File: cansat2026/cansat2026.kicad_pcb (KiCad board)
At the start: 6 copper layers, 96 x 70 mm, 282 parts, among them J101 MCU_UART_Conn, J102 CAM_Conn, J103 MCU_CAM_UART_Conn, J104 I2C_Conn, J105 MCU_Power, J106 MCU_Power, J107 Micro_SD_Card_Det_Hirose_DM3AT, J1101 USB_C_Receptacle_USB2.0_14P, J1102 USB_C_Receptacle_USB2.0_14P, J201 FlightPin, J301 Battery, J302 Battery, J401 M1, J402 M2, J403 M3, J801 Conn_Coaxial, Q1101 2N7002, Q1102 2N7002, Q1103 2N7002, Q1104 2N7002, Q301 2SB1198K, Q302 2SB1198K, Q303 2N7002, Q304 2SB1198K, Q305 2N7002, Q306 2SC2412K, Q307 PJA3404A, Q308 PJA3404A, SW201 SW_SPST, SW901 SW_SPST, U1001 ICE40UP5K-SG48ITR, U101 E220-900T22S(JP), U1101 USBLC6-2SC6, U1102 CH340K, U1103 USBLC6-2SC6, U1104 CH340K, U201 TPS70912DRVR, U202 TCR2LN18, U203 TPS561201DDC, U204 74HC08, U205 INA226, U206 TPS562242, U207 XC6206P332MR, U208 TPS62180, U209 TPS62180, U210 TPS63070, U301 S-8209ABB-T8T1U, U302 S-8209ABB-T8T1U, U401 TC78H653FTG, U402 TC78H653FTG, U403 AM8068, U601 HP203B, U701 LSM6DSV, U801 MAX-M10S, U901 ESP32-S3-WROOM-1U-N4R8, U902 ESP32-S3-WROOM-1U-N4R8, U903 AW9523B, U904 PCA9306DQER, U905 PCA9306DQER

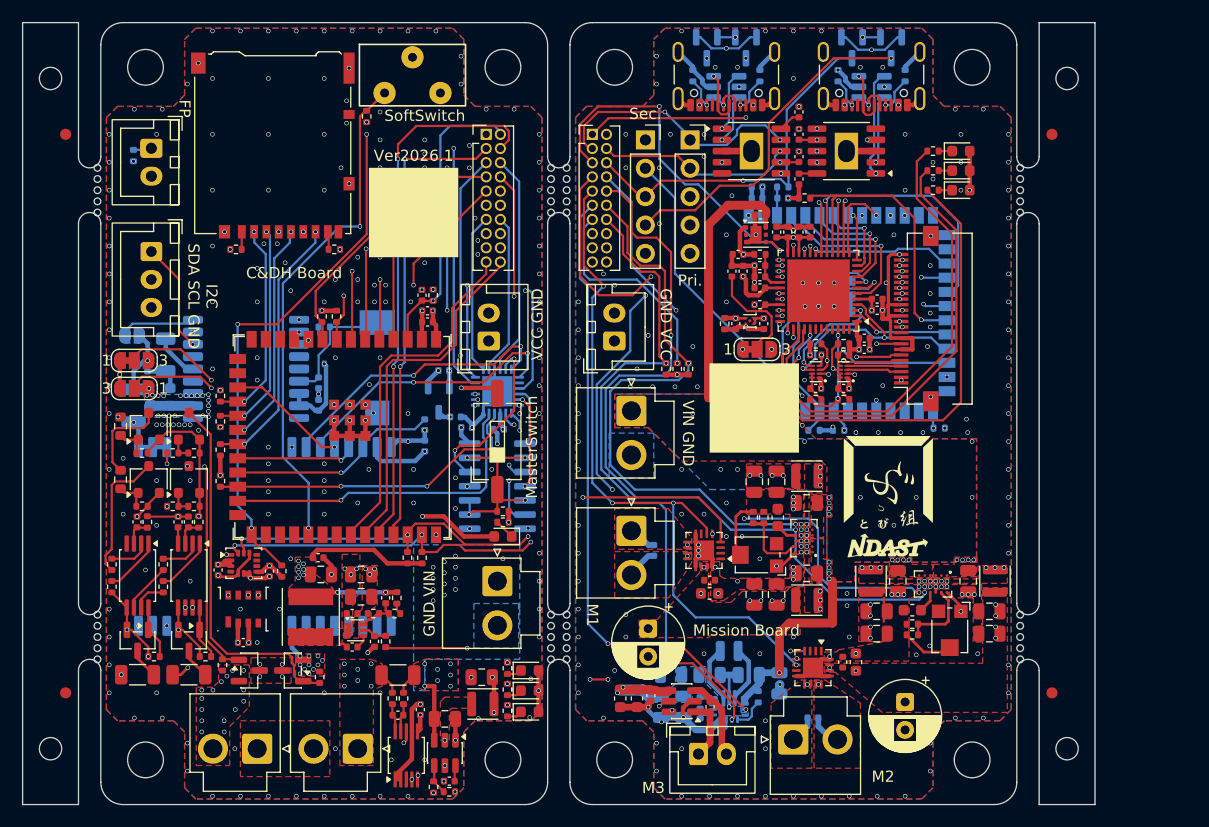
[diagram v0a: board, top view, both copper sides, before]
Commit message: ARLISSに作り直した
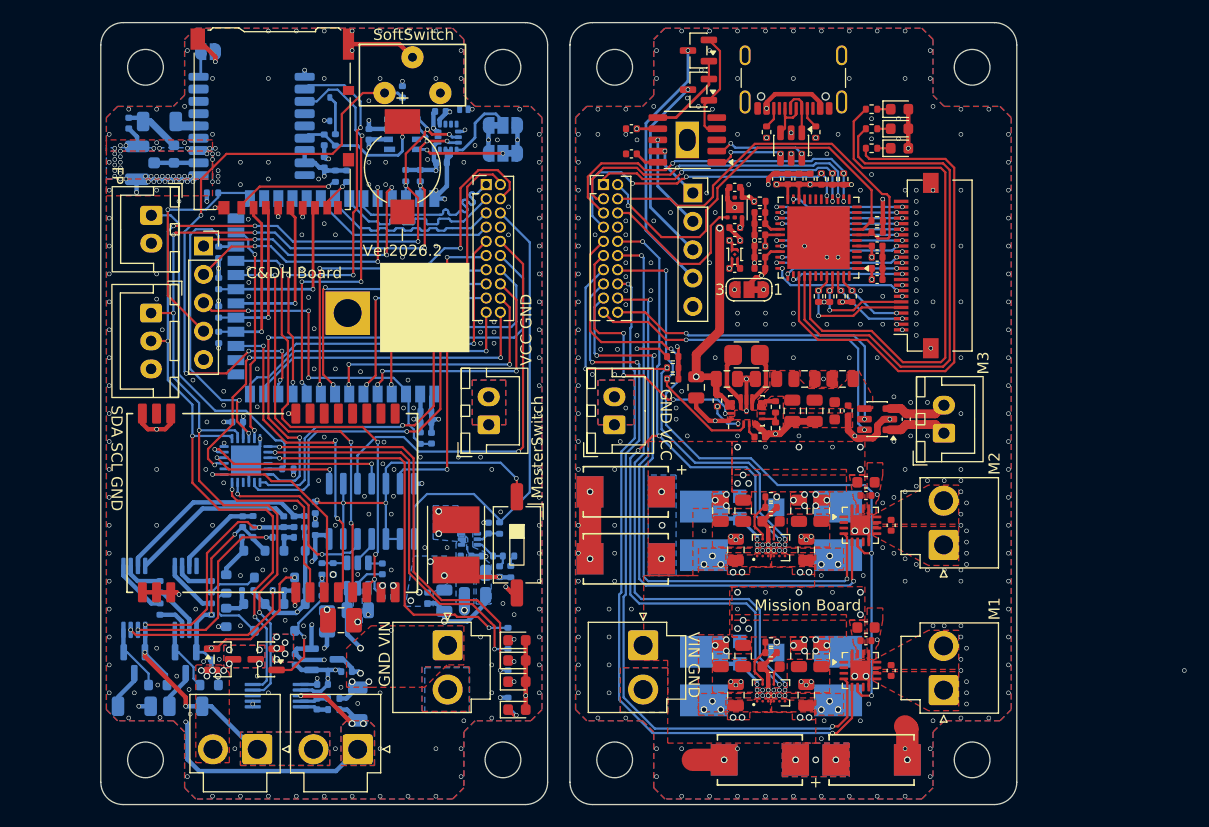
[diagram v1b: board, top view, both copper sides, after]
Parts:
- removed C1103, C1104, C908, C909: 100nF, Capacitor_SMD:C_0402_1005Metric
- removed the C903 at (98.7, 35.5)
- removed the C904 at (98.7, 34.5)
- removed C905: 1uF, Capacitor_SMD:C_0402_1005Metric
- removed the J103 at (88.7, 30.2)
- removed J1102: USB_C_Receptacle_USB2.0_14P, Connector_USB:USB_C_Receptacle_GCT_USB4105-xx-A_16P_TopMnt_Horizontal
- removed Q1103, Q1104: 2N7002, Package_TO_SOT_SMD:SOT-23
- removed R1103, R1104: 5.1k, Resistor_SMD:R_0402_1005Metric
- removed the R901 at (101.0, 34.5)
- removed the R905 at (115.0, 56.0)
- removed the R909 at (59.8, 46.0)
- removed the R917 at (103.0, 35.5)
- removed the R918 at (106.5, 53.5)
- removed the R919 at (95.8, 46.7)
- removed R923: 200k, Resistor_SMD:R_0402_1005Metric
- removed the REF** at (126.5, 24.8)
- removed the REF** at (125.1, 79.8)
- removed the REF** at (36.8, 29.8)
- removed the REF** at (125.1, 29.8)
- removed the REF** at (80.0, 74.8)
- removed the REF** at (40.0, 34.8)
- removed the REF** at (80.0, 34.8)
- removed the REF** at (36.8, 79.8)
- removed the REF** at (122.0, 34.8)
- removed the REF** at (35.5, 84.8)
- removed the REF** at (40.0, 74.8)
- removed the REF** at (126.5, 84.8)
- removed the REF** at (35.5, 24.8)
- removed the REF** at (122.0, 74.8)
- removed U1103: USBLC6-2SC6, Package_TO_SOT_SMD:SOT-23-6
- removed U1104: CH340K, Package_SO:SSOP-10-1EP_3.9x4.9mm_P1mm_EP2.1x3.3mm
- removed the U902 at (106.2, 45.8)
- removed U904, U905: PCA9306DQER, Package_SON:X2SON-8_1.4x1mm_P0.35mm
- added C413: 100uF, Project:MURATA_ECAS_D6, B.Cu at (99.0, 85.8)
- added C414: 100uF, Project:MURATA_ECAS_D6, F.Cu at (87.0, 61.8)
- added C415: 100uF, Project:MURATA_ECAS_D6, B.Cu at (87.0, 61.8)
- added C416: 100uF, Project:MURATA_ECAS_D6, F.Cu at (87.0, 67.8)
- added C417: 100uF, Project:MURATA_ECAS_D6, B.Cu at (87.0, 67.8)
- added C418: 22uF, Capacitor_SMD:C_0805_2012Metric, F.Cu at (106.4, 51.6)
- added J101: MCU_UART_Conn, Connector_PinSocket_2.54mm:PinSocket_1x05_P2.54mm_Vertical, F.Cu at (49.2, 39.8)
- added R906: 10k, Resistor_SMD:R_0402_1005Metric, F.Cu at (105.5, 33.8)
- added R907: 10k, Resistor_SMD:R_0402_1005Metric, F.Cu at (104.5, 33.8)
- BT801, C235, C236, C237, C238, C239, C240, C241, C403, C406, Q1101, Q1102, R1002, R1003, R1101, R1102, R220, R221, R222, U101, U1101, U210: moved to F.Cu
- C205, C206, C207, C209, C210, C211, C212, C213, C214, C215, C216, C217, C218, C301, C302, C303, C601, C701, C702, C901, C902, G*** (x2), JP601, JP701, Q301, Q302, Q303, Q304, Q305, Q306, R101, R102, R202, R203, R204, R205, R206, R207, R208, R209, R210, R211, R218, R301, R302, R303, R304, R305, R306, R308, R309, R310, R311, R312, R313, R315, R316, R317, R318, R319, R320, RV201, RV202, U203, U205, U206, U301, U302, U601, U701, U901: moved to B.Cu
- C410: footprint Capacitor_THT:CP_Radial_D6.3mm_P2.50mm -> Project:MURATA_ECAS_D6
- C411: footprint Capacitor_THT:CP_Radial_D6.3mm_P2.50mm -> Project:MURATA_ECAS_D6; moved to B.Cu
- C412: value 10uF -> 100uF; footprint Capacitor_SMD:C_0603_1608Metric -> Project:MURATA_ECAS_D6
- C903: renamed from C906; moved to B.Cu
- L201: footprint Inductor_SMD:L_Wuerth_PMCI-252012 -> Inductor_SMD:L_1008_2520Metric_Pad1.43x2.20mm_HandSolder
- L202: footprint Inductor_SMD:L_Taiyo-Yuden_NR-50xx -> Inductor_SMD:L_Taiyo-Yuden_NR-50xx_HandSoldering
- L203, L204, L205, L206: footprint Inductor_SMD:L_Wuerth_PMCI-252010 -> Project:L_Taiyo-Yuden_LSEU-4040; moved to B.Cu
- L207: footprint Inductor_SMD:L_Wuerth_PMCI-201610 -> Project:L_Wuerth_PMCI-201610; moved to F.Cu
- R307, R314: footprint Resistor_SMD:R_0402_1005Metric -> Resistor_SMD:R_0603_1608Metric; moved to B.Cu
- R901: renamed from R902; moved to B.Cu
- R902: renamed from R903; moved to B.Cu
- R903: renamed from R904; moved to B.Cu
- R904: renamed from R906; moved to B.Cu
- R905: renamed from R907; moved to B.Cu
- R908: value 4.7k -> 10k
- R909: renamed from R911; moved to B.Cu
- R910: renamed from R912; moved to B.Cu
- R911: renamed from R913; moved to B.Cu
- R914: renamed from R910; moved to B.Cu
- R917: renamed from R914; moved to B.Cu
- R918: renamed from R915; moved to B.Cu
- R919: renamed from R916; moved to B.Cu
- moved R908 47.0 mm to (106.5, 33.8), turned to 90 degrees
- moved C601 46.9 mm to (64.0, 29.8), turned to -90 degrees
- moved U601 44.8 mm to (67.0, 29.8), turned to 90 degrees
- moved C702 43.9 mm to (70.4, 27.7), turned to 180 degrees
- moved U701 42.3 mm to (71.1, 30.0), turned to 90 degrees
- moved C701 41.6 mm to (70.5, 32.3), turned to 0 degrees
- moved JP601 39.1 mm to (76.0, 31.4)
- moved JP701 39.1 mm to (76.0, 28.9)
- moved J403 36.2 mm to (115.4, 56.5), turned to 90 degrees
- moved R903 34.4 mm to (50.0, 35.0), turned to 0 degrees
- moved R904 34.2 mm to (68.6, 33.5), turned to -90 degrees
- moved R905 34.2 mm to (67.3, 33.5), turned to -90 degrees
- moved J401 31.4 mm to (115.4, 79.5), turned to 90 degrees
- moved R201 31.3 mm to (56.7, 59.7), turned to 180 degrees
- moved C407 31.2 mm to (105.7, 54.5)
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- renumbered C907 to C904, J104 to J103, J105 to J104, J106 to J105, J107 to J106, R920 to R912, R921 to R913, R924 to R915, R925 to R916, U903 to U902
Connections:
- C1011 pad 1: /VCC -> Net-(JP1001-C)
- C1012 pad 1: /VCC -> Net-(JP1001-C)
- C411 pad 1: /MD/M2PWR -> /MD/M1PWR
- C412 pad 1: /MD/M3PWR -> /MD/M1PWR
- R908 pad 2: /MCU/I2C2SDA -> /MCU/FPGA_SPI_MISO
- R912 pad 2: /MCU/CP_CAM_PIN_SIOC -> /CAM_PIN_SIOC
- R913 pad 2: /MCU/CP_CAM_PIN_SIOD -> /CAM_PIN_SIOD
- REF** pad 1: /GPIO0 -> /MCU/FPGA_SPI_SS (x2)
- REF** pad 2: /EN -> /MCU/FPGA_~{CRESET} (x2)
- REF** pad 3: /U0TXD -> /MCU/FPGA_SPI_SCK (x2)
- REF** pad 4: /U0RXD -> /MCU/FPGA_CDONE (x2)
- REF** pad 5: /Power/MASTER_EN -> /MCU/FPGA_SPI_MISO (x2)
- REF** pad 6: /MCU_CAM_EN -> /Power/MASTER_EN (x2)
- REF** pad 7: /MCU/I2C2SCL -> /MCU/FPGA_SPI_MOSI (x2)
- REF** pad 8: /MCU/I2C2SDA -> (no net) (x2)
- U1001 pad 1: /VCC -> Net-(JP1001-C)
- U1001 pad 10: /MCU/CP_CAM_PIN_D2 -> unconnected-(U1001B-IOB_18a-Pad10)
- U1001 pad 11: /MCU/CP_CAM_PIN_D3 -> unconnected-(U1001B-IOB_20a-Pad11)
- U1001 pad 12: /MCU/CP_CAM_PIN_D4 -> unconnected-(U1001B-IOB_22a-Pad12)
- U1001 pad 13: /MCU/CP_CAM_PIN_D6 -> unconnected-(U1001B-IOB_24a-Pad13)
- U1001 pad 18: /MCU/CP_CAM_PIN_D7 -> unconnected-(U1001B-IOB_31b-Pad18)
- U1001 pad 19: /MCU/CP_CAM_PIN_HREF -> unconnected-(U1001B-IOB_29b-Pad19)
- U1001 pad 2: /MCU/CP_CAM_PIN_VSYNC -> unconnected-(U1001C-IOB_6a-Pad2)
- U1001 pad 20: /MCU/CP_CAM_PIN_PCLK -> unconnected-(U1001B-IOB_25b_G3-Pad20)
- U1001 pad 21: /MCU/CP_CAM_PIN_D5 -> unconnected-(U1001B-IOB_23b-Pad21)
- U1001 pad 3: /MCU/CP_CAM_PIN_RESET -> unconnected-(U1001C-IOB_9b-Pad3)
- U1001 pad 4: /MCU/CP_CAM_PIN_PWDN -> unconnected-(U1001C-IOB_8a-Pad4)
- U1001 pad 44: unconnected-(U1001C-IOB_3b_G6-Pad44) -> /CAM_PIN_PWDN
- U1001 pad 45: unconnected-(U1001C-IOB_5b-Pad45) -> /CAM_PIN_RESET
- U1001 pad 46: /MCU/LS_EN -> /CAM_PIN_SIOC
- U1001 pad 47: unconnected-(U1001C-IOB_2a-Pad47) -> /CAM_PIN_SIOD
- U1001 pad 6: /MCU/CP_CAM_PIN_D0 -> unconnected-(U1001B-IOB_13b-Pad6)
- U1001 pad 9: /MCU/CP_CAM_PIN_D1 -> unconnected-(U1001B-IOB_16a-Pad9)
- U210 pad : VIN -> (no net)
- U801 pad 16: /I2C1SDA -> unconnected-(U801-SDA-Pad16)
- U801 pad 17: /I2C1SCL -> unconnected-(U801-SCL-Pad17)
- U901 pad 12: unconnected-(U901-GPIO8/TOUCH8/ADC1_CH7/SUBSPICS1-Pad12) -> /MCU/SW_SOFT
- U901 pad 13: unconnected-(U901-GPIO19/U1RTS/ADC2_CH8/CLK_OUT2/USB_D--Pad13) -> /MCU/MC2
- U901 pad 14: unconnected-(U901-GPIO20/U1CTS/ADC2_CH9/CLK_OUT1/USB_D+-Pad14) -> /MCU/MC1
- U901 pad 31: /MCU/SW_SOFT -> unconnected-(U901-GPIO38/FSPIWP/SUBSPIWP-Pad31)
- U901 pad 32: unconnected-(U901-MTCK/GPIO39/CLK_OUT3/SUBSPICS1-Pad32) -> /MCU/FPGA_SPI_MOSI
- U901 pad 33: unconnected-(U901-MTDO/GPIO40/CLK_OUT2-Pad33) -> /MCU/FPGA_SPI_MISO
- U901 pad 34: /MCU/MC1 -> /MCU/FPGA_SPI_SCK
- U901 pad 35: /MCU/MC2 -> /MCU/FPGA_SPI_SS
- U901 pad 8: /MCU/I2C2SDA -> /MCU/FPGA_~{CRESET}
- U901 pad 9: /MCU/I2C2SCL -> /MCU/FPGA_CDONE
- U902 pad 10: /MCU_CAM_EN -> unconnected-(U902-P0_4-Pad10)
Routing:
- net GND: track 225.1 -> 419.4 mm, vias 434 -> 573
- net /MCU_CAM_GPIO0: track 67.8 -> 0.00 mm, vias 2 -> 0
- net /MCU/I2C2SCL: track 60.2 -> 0.00 mm, vias 2 -> 0
- net /MCU/I2C2SDA: track 57.4 -> 0.00 mm, vias 4 -> 0
- net /MCU_CAM_EN: track 53.1 -> 0.00 mm, vias 1 -> 0
- net /MCU/FPGA_CDONE: track 22.4 -> 73.7 mm, vias 1 -> 3
- net /MCU_CAM_U0RXD: track 51.0 -> 0.00 mm, vias 2 -> 0
- net /MCU/FPGA_~{CRESET}: track 26.4 -> 72.3 mm, vias 3 -> 4
- net /GPIO0: track 89.4 -> 44.4 mm, vias 5 -> 2
- net /MCU_CAM_U0TXD: track 43.7 -> 0.00 mm, vias 2 -> 0
- net Net-(U210-EN): track 90.3 -> 52.7 mm, vias 5 -> 6
- net /GPS/GPS_TX: track 0.83 -> 38.2 mm, vias 1 -> 4
- net /GPS/GPS_RX: track 0.99 -> 37.1 mm, vias 1 -> 4
- net /3.8V: track 45.5 -> 9.46 mm, vias 4 -> 3
- net /U0TXD: track 65.2 -> 29.3 mm
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- added copper zone on In2.Cu, net /1.2V
- added copper zone on B.Cu, net /MD/M1PWR
- added copper zone on B.Cu, net /MD/M2PWR
- added copper zone on F.Cu, net /MD/M3PWR
- added copper zone on B.Cu, net /Power/BATT+
- added copper zone on In1.Cu, net /Power/BATT+
- added copper zone on B.Cu, net /VCC
- added copper zone on B.Cu, net Net-(J301-Pin_2)
- added copper zone on In1.Cu, net Net-(J301-Pin_2)
- added copper zone on In2.Cu, net Net-(J302-Pin_2)
- added copper zone on In2.Cu, net Net-(JP1001-C)
- added copper zone on B.Cu, net Net-(Q307-D)
- added copper zone on In2.Cu, net Net-(Q307-D)
- added copper zone on B.Cu, net Net-(U203-SW)
- added copper zone on B.Cu, net Net-(U206-SW)
- removed copper zone on In3.Cu, net /MD/M1PWR
- removed copper zone on In3.Cu, net /MD/M2PWR
- removed copper zone on B.Cu, net /MD/M3PWR
- removed copper zone on F.Cu, net /VCC
- removed copper zone on In3.Cu, net GND
- removed copper zone on In4.Cu, net GND
- removed copper zone on In4.Cu, net Net-(J301-Pin_2)
- removed copper zone on In2.Cu, net Net-(J401-Pin_1)
- removed copper zone on In2.Cu, net Net-(J401-Pin_2)
- removed copper zone on In2.Cu, net Net-(J402-Pin_1)
- removed copper zone on In2.Cu, net Net-(J402-Pin_2)
- removed copper zone on F.Cu, net Net-(U203-SW)
- removed copper zone on F.Cu, net Net-(U206-SW)
- removed copper zone on In3.Cu, net VIN
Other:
- board size 96 x 70 mm -> 82 x 70 mm
- copper layers 6 -> 4
- board text added: "+"
- board text added: "SDA SCL GND"
- board text added: "Ver2026.2"
- board text removed: "I2C SDA SCL GND"
- board text removed: "Pri."
- board text removed: "Sec."
- board text removed: "Ver2026.1"
